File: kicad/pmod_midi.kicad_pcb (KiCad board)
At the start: 2 copper layers, 24 x 45.6 mm, 17 parts, among them J1 PMOD (12 Pin), J2 Conn_01x02_Pin, J3 CME_Widi_Core_1-8, J4 CME_Widi_Core_9-16, Q1 Q_NPN_BCE

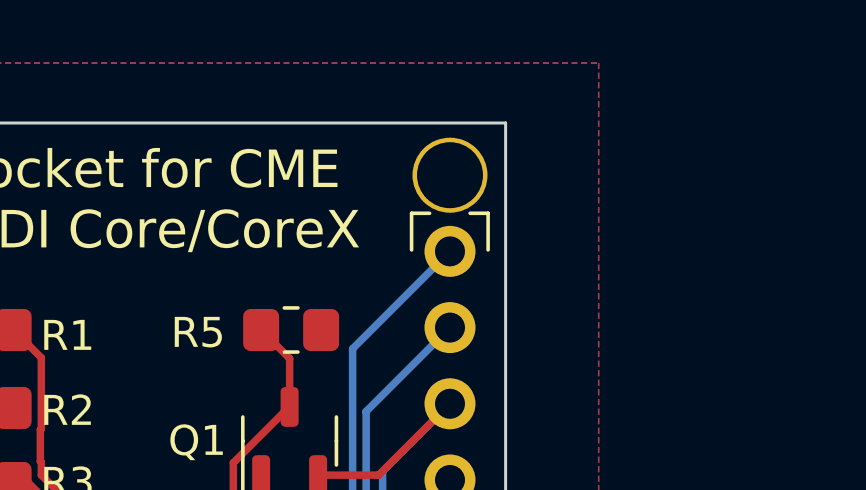
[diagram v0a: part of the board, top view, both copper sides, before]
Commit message: Updated BOM
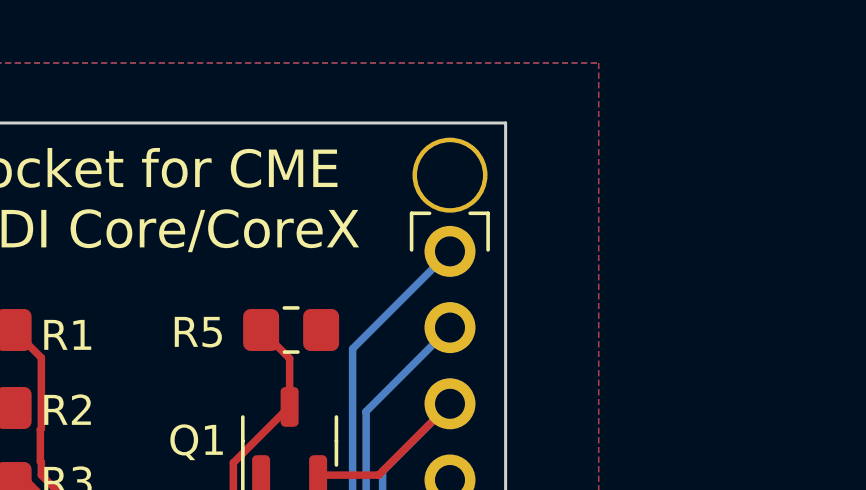
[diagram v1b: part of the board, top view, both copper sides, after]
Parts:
- removed the REF** at (122.0, 41.6)
- removed the REF** at (101.7, 41.7)
- added H1: MountingHole_Pad, CME:Standoff Spacer, F.Cu at (101.7, 41.7)
- added H2: MountingHole_Pad, CME:Standoff Spacer, F.Cu at (122.0, 41.6)
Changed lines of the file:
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@@
   (net 21 "/RED")
   (net 22 "/BT*")
-  (footprint "CME:Standoff Spacer" (layer "F.Cu")
-    (at 122.025938 41.61975)
-    (attr through_hole board_only)
-    (fp_text reference "REF**" (at 0.43 -2.35 unlocked) (layer "F.SilkS") hide
-        (effects (font (size 1 1) (thickness 0.15)))
-    )
-    (fp_text value "Standoff Spacer" (at 0 1 unlocked) (layer "F.Fab") hide
-        (effects (font (size 1 1) (thickness 0.15)))
-    )
-    (fp_text user "${REFERENCE}" (at 0 2.5 unlocked) (layer "F.Fab") hide
-        (effects (font (size 1 1) (thickness 0.15)))
-    )
-    (fp_circle (center 0.12 0.120354) (end 0.15 -1.149646)
-      (stroke (width 0.05) (type default)) (fill none) (layer "F.CrtYd"))
-    (pad "1" thru_hole circle (at 0.12 0.12) (size 2.5 2.5) (drill 2.2) (layers "*.Cu" "*.Mask")
-      (net 8 "/GND"))
-  )
   (footprint "Resistor_SMD:R_0805_2012Metric_Pad1.20x1.40mm_HandSolder" (layer "F.Cu")
     (at 116.85 57.1)
@@
       (net 7 "/3.3V") (pinfunction "VCC") (pintype "passive"))
   )
-  (footprint "CME:Standoff Spacer" (layer "F.Cu")
-    (at 101.745938 41.65375)
-    (attr through_hole board_only)
-    (fp_text reference "REF**" (at 0.43 -2.35 unlocked) (layer "F.SilkS") hide
-        (effects (font (size 1 1) (thickness 0.15)))
-    )
-    (fp_text value "Standoff Spacer" (at 0 1 unlocked) (layer "F.Fab") hide
-        (effects (font (size 1 1) (thickness 0.15)))
-    )
-    (fp_text user "${REFERENCE}" (at 0 2.5 unlocked) (layer "F.Fab") hide
-        (effects (font (size 1 1) (thickness 0.15)))
-    )
-    (fp_circle (center 0.12 0.120354) (end 0.15 -1.149646)
-      (stroke (width 0.05) (type default)) (fill none) (layer "F.CrtYd"))
-    (pad "1" thru_hole circle (at 0.12 0.12) (size 2.5 2.5) (drill 2.2) (layers "*.Cu" "*.Mask")
-      (net 8 "/GND"))
-  )
   (footprint "Button_Switch_THT:SW_PUSH_6mm" (layer "F.Cu")
     (at 109.9 66.7 -90)
@@
     (property "MPN" "SSW-108-01-L-S")
     (property "Manufacturer" "Samtec")
-    (property "Notes" "1x8 0.1 Inch pitch pin header socket; Optional: 11mm M2 female to female standoff spacer, Two plastic/nylon m2 pan head bolts. For insertion of pins 9-16 of [CME Widi Core module](https://www.cme-pro.com/wp-content/uploads/2022/10/widiCore-Doc-v1.3.pdf).")
+    (property "Notes" "1x8 0.1 Inch pitch pin header socket; . For insertion of pins 9-16 of [CME Widi Core module](https://www.cme-pro.com/wp-content/uploads/2022/10/widiCore-Doc-v1.3.pdf).")
     (property "Sheetfile" "pmod_midi.kicad_sch")
     (property "Sheetname" "")
@@
     (property "MPN" "SSW-108-01-L-S")
     (property "Manufacturer" "Samtec")
-    (property "Notes" "1x8 0.1 Inch pitch pin header socket; Optional: 11mm M2 female to female standoff spacer, Two plastic/nylon m2 pan head bolts. For insertion of pins 1-8 of [CME Widi Core module](https://www.cme-pro.com/wp-content/uploads/2022/10/widiCore-Doc-v1.3.pdf).")
+    (property "Notes" "1x8 0.1 Inch pitch pin header socket; . For insertion of pins 1-8 of [CME Widi Core module](https://www.cme-pro.com/wp-content/uploads/2022/10/widiCore-Doc-v1.3.pdf).")
     (property "Sheetfile" "pmod_midi.kicad_sch")
     (property "Sheetname" "")
@@
     )
   )
+  (footprint "CME:Standoff Spacer" (layer "F.Cu")
+    (at 122.025938 41.619396)
+    (property "MPN" "970100244")
+    (property "Manufacturer" "Würth Elektronik")
+    (property "Notes" "Optional: 10mm M2 female to female standoff spacer, ")
+    (property "Sheetfile" "pmod_midi.kicad_sch")
+    (property "Sheetname" "")
+    (property "ki_description" "Mounting Hole with connection")
+    (property "ki_keywords" "mounting hole")
+    (attr through_hole)
+    (fp_text reference "H2" (at 0.43 -2.35 unlocked) (layer "F.SilkS") hide
+        (effects (font (size 1 1) (thickness 0.15)))
+    )
+    (fp_text value "MountingHole_Pad" (at 0 1 unlocked) (layer "F.Fab") hide
+        (effects (font (size 1 1) (thickness 0.15)))
+    )
+    (fp_text user "${REFERENCE}" (at 0 2.5 unlocked) (layer "F.Fab") hide
+        (effects (font (size 1 1) (thickness 0.15)))
+    )
+    (fp_circle (center 0.12 0.120354) (end 0.15 -1.149646)
+      (stroke (width 0.05) (type default)) (fill none) (layer "F.CrtYd"))
+    (pad "1" thru_hole circle (at 0.12 0.12) (size 2.5 2.5) (drill 2.2) (layers "*.Cu" "*.Mask")
+      (net 8 "/GND") (pinfunction "1") (pintype "input"))
+  )
+  (footprint "CME:Standoff Spacer" (layer "F.Cu")
+    (at 101.745938 41.65375)
+    (property "MPN" "970100244")
+    (property "Manufacturer" "Würth Elektronik")
+    (property "Notes" "Optional: 10mm M2 female to female standoff spacer, ")
+    (property "Sheetfile" "pmod_midi.kicad_sch")
+    (property "Sheetname" "")
+    (property "ki_description" "Mounting Hole with connection")
+    (property "ki_keywords" "mounting hole")
+    (attr through_hole)
+    (fp_text reference "H1" (at 0.43 -2.35 unlocked) (layer "F.SilkS") hide
+        (effects (font (size 1 1) (thickness 0.15)))
+    )
+    (fp_text value "MountingHole_Pad" (at 0 1 unlocked) (layer "F.Fab") hide
+        (effects (font (size 1 1) (thickness 0.15)))
+    )
+    (fp_text user "${REFERENCE}" (at 0 2.5 unlocked) (layer "F.Fab") hide
+        (effects (font (size 1 1) (thickness 0.15)))
+    )
+    (fp_circle (center 0.12 0.120354) (end 0.15 -1.149646)
+      (stroke (width 0.05) (type default)) (fill none) (layer "F.CrtYd"))
+    (pad "1" thru_hole circle (at 0.12 0.12) (size 2.5 2.5) (drill 2.2) (layers "*.Cu" "*.Mask")
+      (net 8 "/GND") (pinfunction "1") (pintype "input"))
+  )
   (footprint "Symbol:OSHW-Logo2_7.3x6mm_SilkScreen" (layer "B.Cu")
